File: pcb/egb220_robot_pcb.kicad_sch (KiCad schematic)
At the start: 5 parts, among them J1 Conn_01x03_Pin, Q1 SFH309

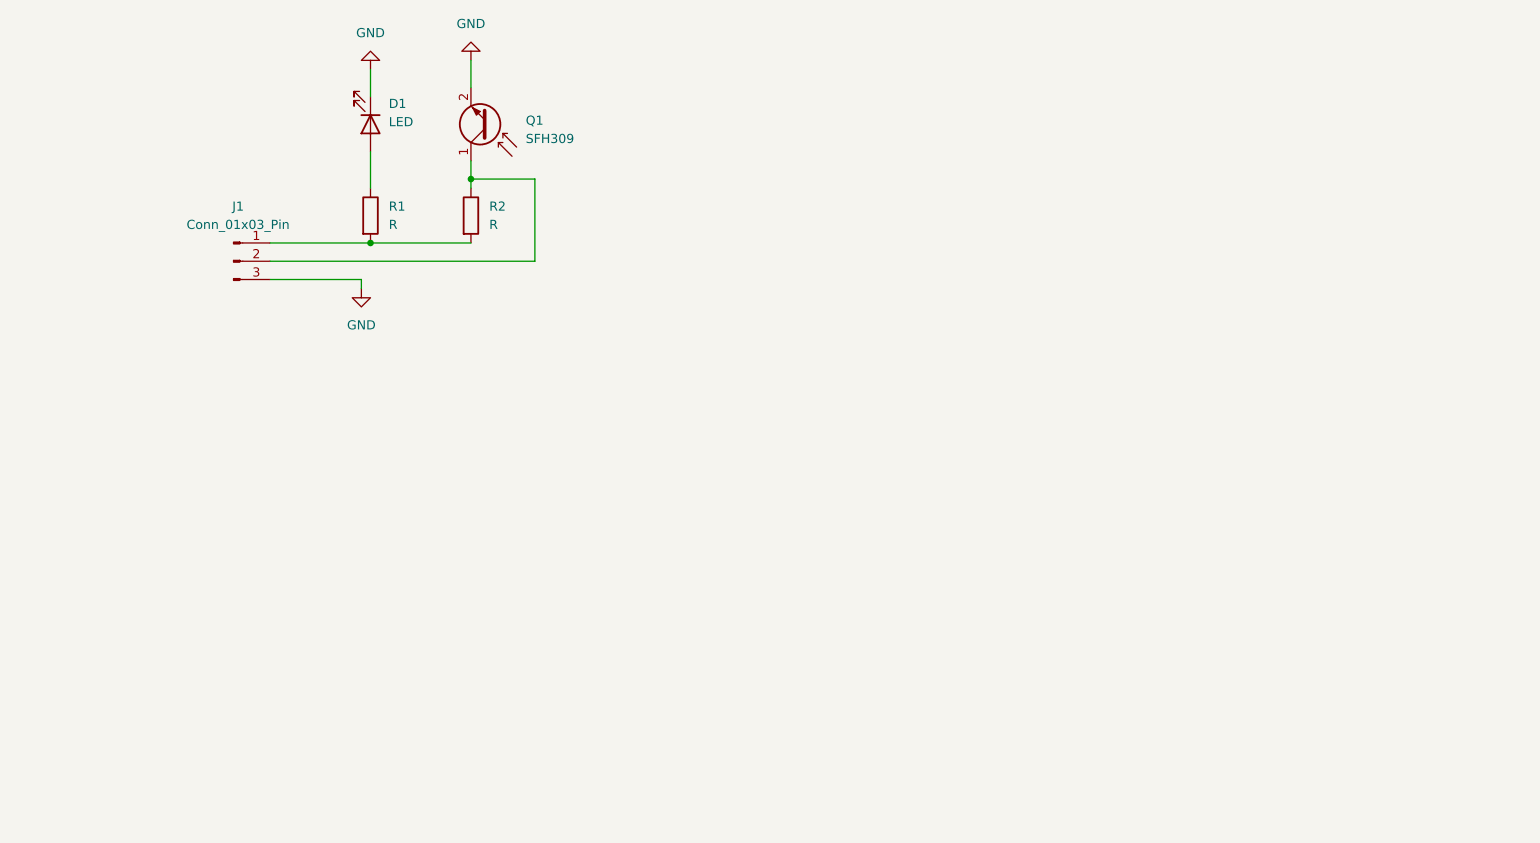
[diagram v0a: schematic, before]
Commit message: feat(PCB): Completed sensor array and first submission
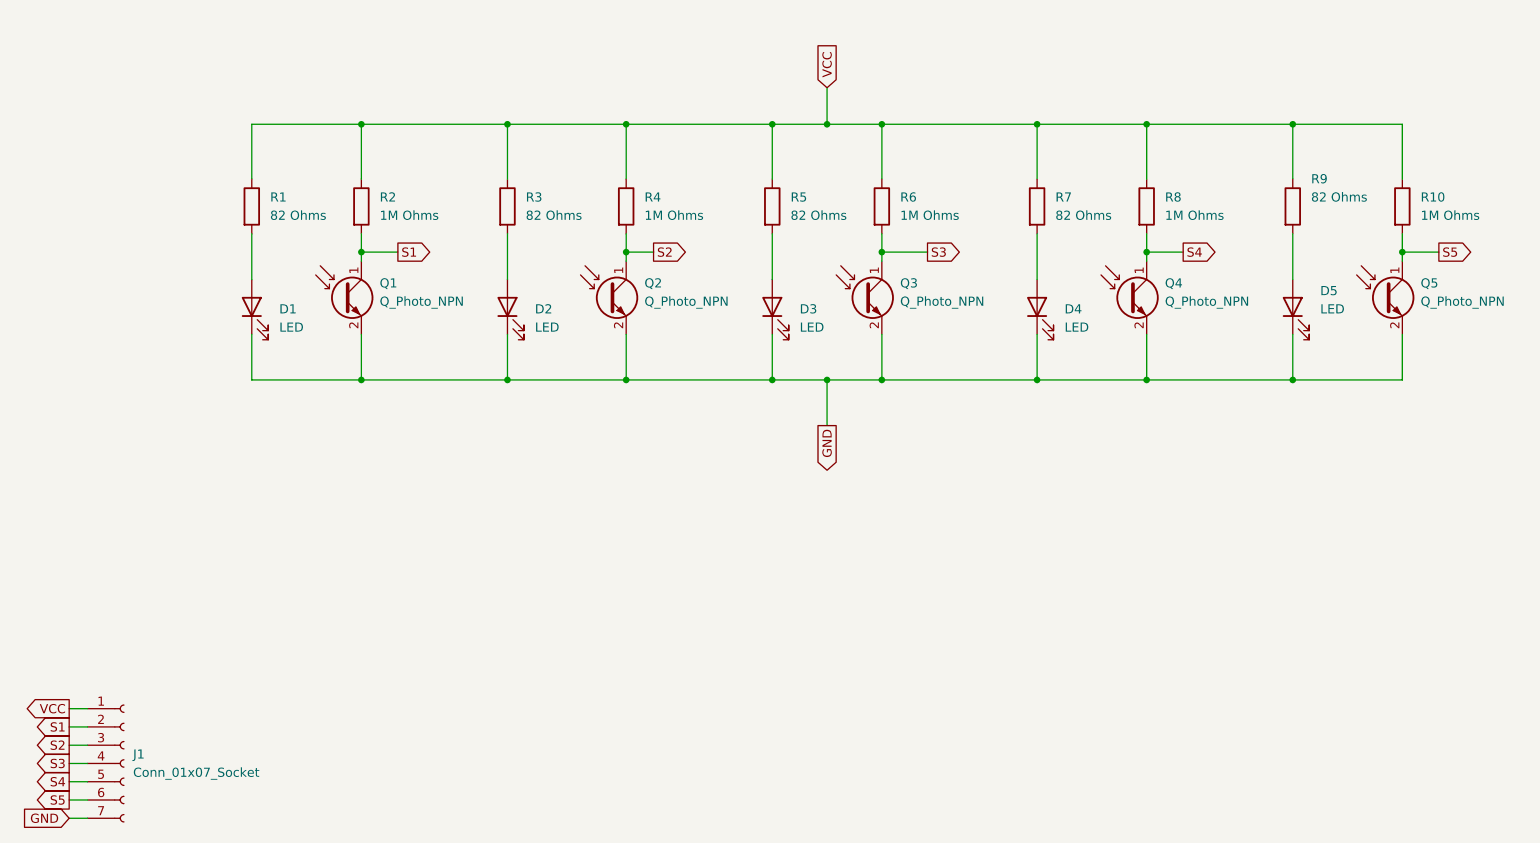
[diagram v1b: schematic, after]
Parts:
- removed J1: Conn_01x03_Pin, Connector_PinHeader_1.27mm:PinHeader_1x03_P1.27mm_Vertical, symbol Connector:Conn_01x03_Pin
- removed Q1: SFH309, LED_THT:LED_D3.0mm_Clear, symbol Sensor_Optical:SFH309
- added D2, D3, D4, D5: LED, LED_THT:LED_D3.0mm_IRGrey, symbol Device:LED
- added J1: Conn_01x07_Socket, Connector_PinSocket_2.54mm:PinSocket_2x04_P2.54mm_Vertical, symbol Connector:Conn_01x07_Socket
- added Q1, Q2, Q3, Q4, Q5: Q_Photo_NPN, LED_THT:LED_D3.0mm_IRBlack, symbol Device:Q_Photo_NPN
- added R10, R4, R6, R8: 1M Ohms, Resistor_SMD:R_0603_1608Metric_Pad0.98x0.95mm_HandSolder, symbol Device:R
- added R3, R5, R7, R9: 82 Ohms, Resistor_SMD:R_0603_1608Metric_Pad0.98x0.95mm_HandSolder, symbol Device:R
- D1: footprint LED_THT:LED_D3.0mm -> LED_THT:LED_D3.0mm_IRGrey
- R1: value R -> 82 Ohms; footprint Resistor_SMD:R_0201_0603Metric -> Resistor_SMD:R_0603_1608Metric_Pad0.98x0.95mm_HandSolder
- R2: value R -> 1M Ohms; footprint Resistor_SMD:R_0402_1005Metric_Pad0.72x0.64mm_HandSolder -> Resistor_SMD:R_0603_1608Metric_Pad0.98x0.95mm_HandSolder
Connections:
- net GND: now also D2.1 (K), D3.1 (K), D4.1 (K), D5.1 (K), J1.7 (Pin_7), Q1.2 (E), Q2.2 (E), Q3.2 (E), Q4.2 (E), Q5.2 (E)
- net at D1.2 (A): now also R1.2; no longer R1.1
- net VCC: now reaches R2.1
- net VCC: now also R1.1, J1.1 (Pin_1), R10.1, R3.1, R4.1, R5.1, R6.1, R7.1, R8.1, R9.1
- net S1: now reaches R2.2
- net S1: now also J1.2 (Pin_2), Q1.1 (C); no longer R1.2
- new net: D5.2 (A), R9.2
- new net: D2.2 (A), R3.2
- new net: D4.2 (A), R7.2
- new net: D3.2 (A), R5.2
- new net S2: J1.3 (Pin_3), Q2.1 (C), R4.2
- new net S3: J1.4 (Pin_4), Q3.1 (C), R6.2
- new net S4: J1.5 (Pin_5), Q4.1 (C), R8.2
- new net S5: J1.6 (Pin_6), Q5.1 (C), R10.2
